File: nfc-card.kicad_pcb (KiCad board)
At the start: 2 copper layers, 85.6 x 54 mm, 5 parts, among them U1 NT3H2111W0FHKH

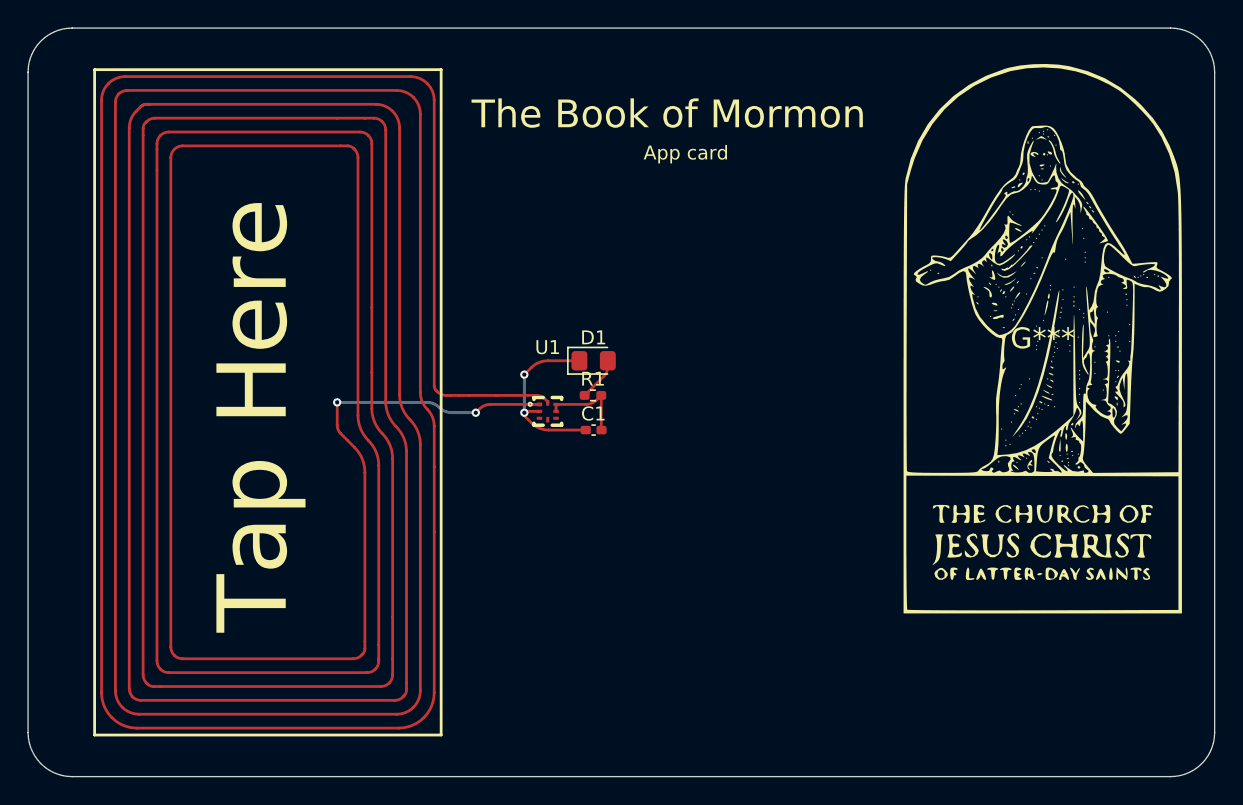
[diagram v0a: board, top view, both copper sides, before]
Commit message: finnished readme and set up production files for jlcpcb
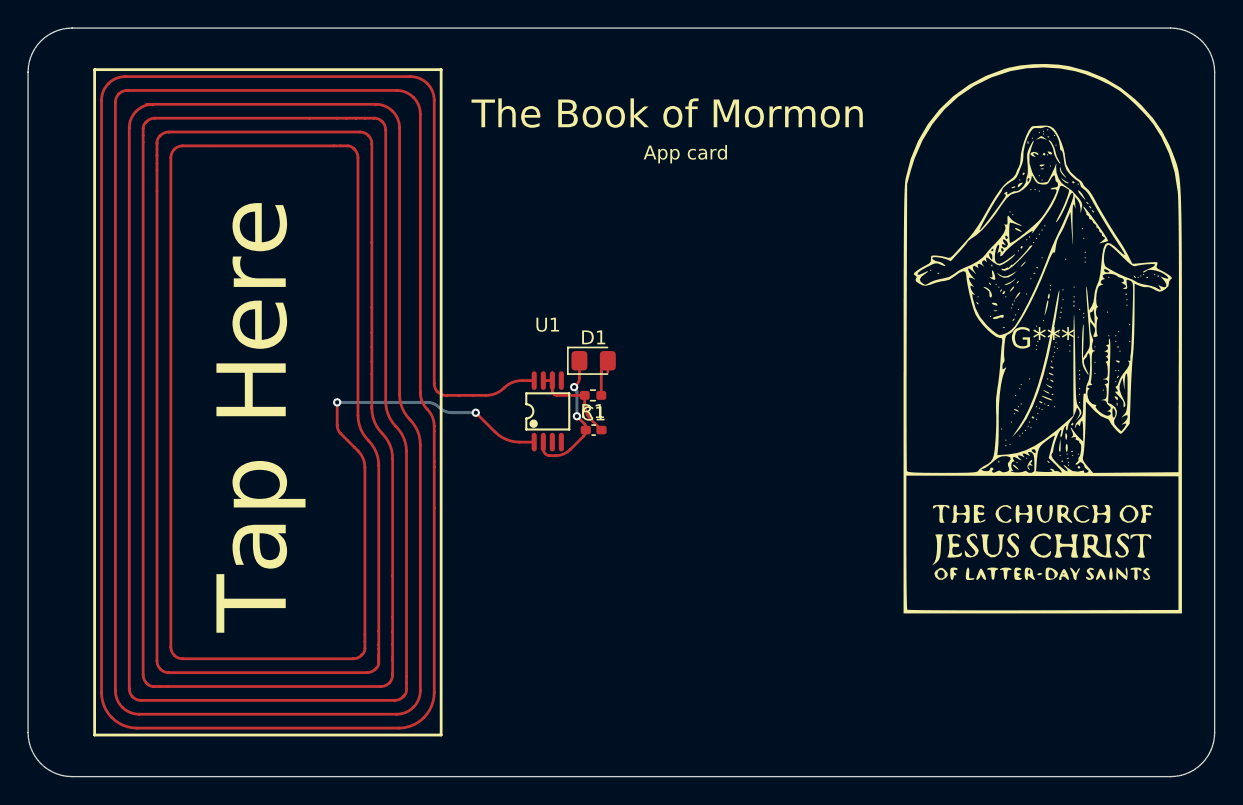
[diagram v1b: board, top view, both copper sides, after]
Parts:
- added G***: LOGO, LOGO, B.Cu at (92.4, 72.2)
- U1: footprint easyeda2kicad:XQFN-8_L1.6-W1.6-P0.50-BL_NT3H2111W0FHKH -> easyeda2kicad:TSSOP-8_L3.0-W3.0-P0.65-LS4.9-BL
- turned R1 to 180 degrees
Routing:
- net Net-(D1-K): track 13.2 -> 10.1 mm
- net Net-(U1-LA): track 742.7 -> 741.4 mm
